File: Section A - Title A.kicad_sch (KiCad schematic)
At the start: 37 parts, among them Q1 SI2303CDS-T1-GE3, U1 AD7190WBRUZ, Y2 CSTCR4M91G53-R0

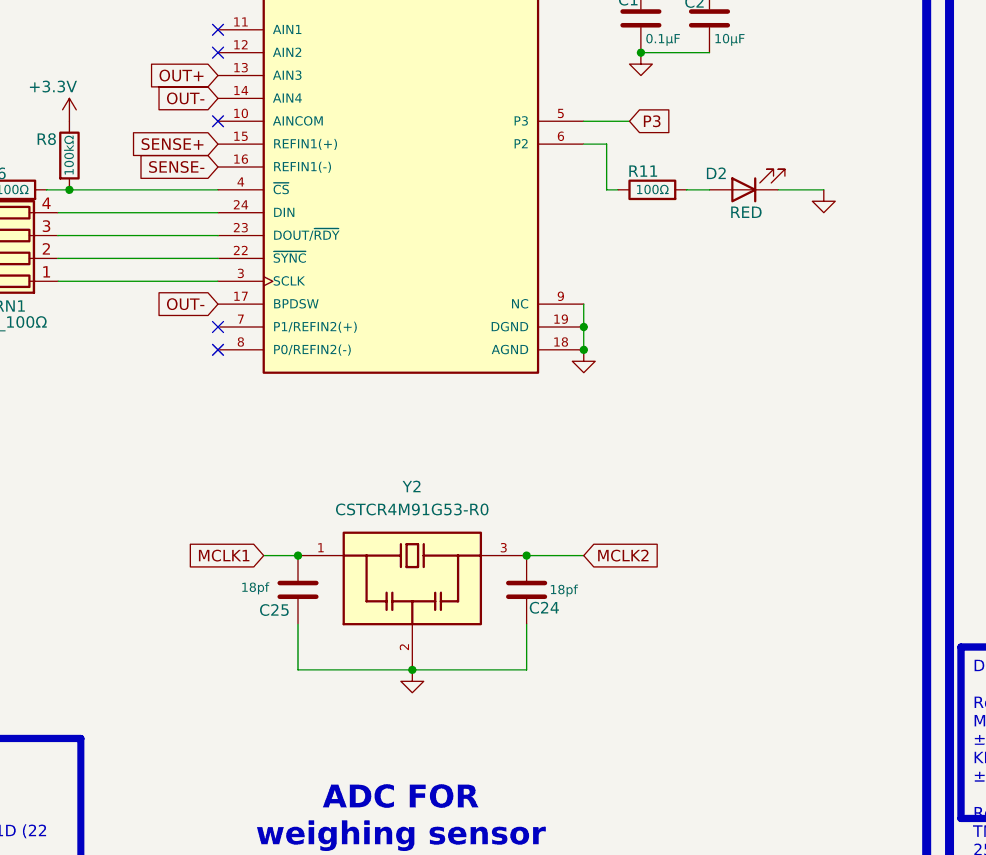
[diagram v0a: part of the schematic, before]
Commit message: [PCB V3]
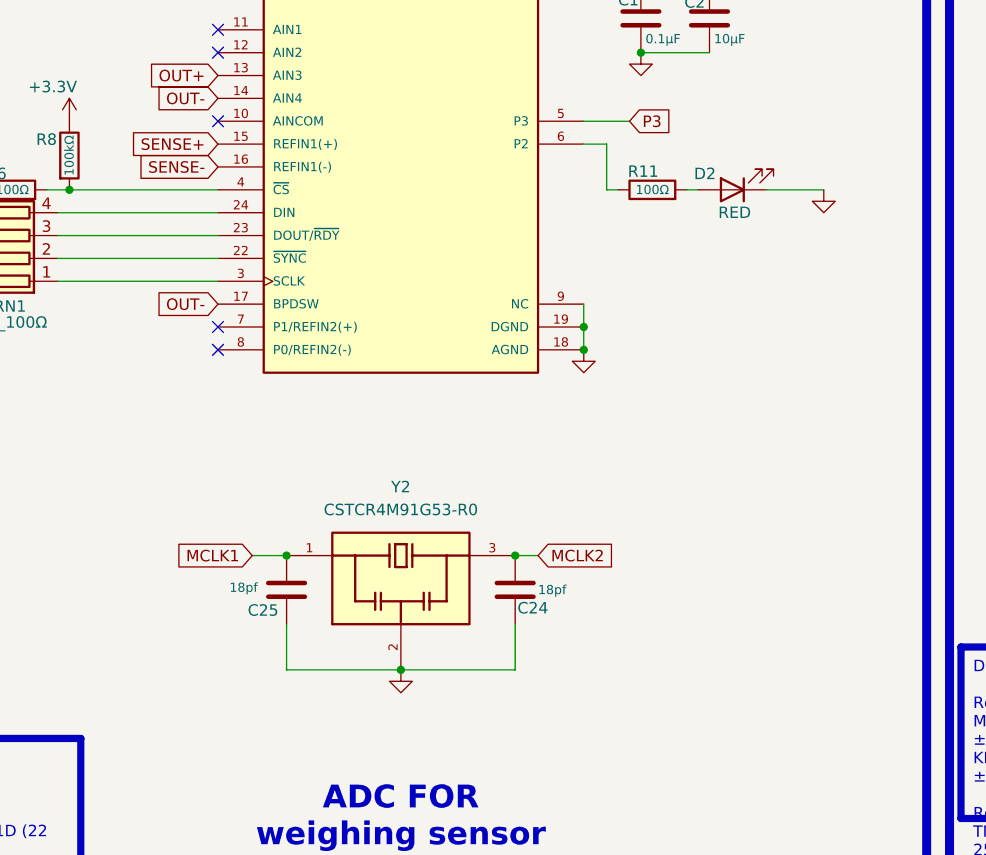
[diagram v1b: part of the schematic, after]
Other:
- moved on the sheet: C24, C25, D2, Y2
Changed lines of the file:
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@@
 	)
 	(junction
-		(at 100.33 125.73)
+		(at 99.06 125.73)
 		(diameter 0)
 		(color 0 0 0 0)
@@
 	)
 	(junction
-		(at 113.03 113.03)
+		(at 111.76 113.03)
 		(diameter 0)
 		(color 0 0 0 0)
@@
 	)
 	(junction
-		(at 87.63 113.03)
+		(at 86.36 113.03)
 		(diameter 0)
 		(color 0 0 0 0)
@@
 	(wire
 		(pts
-			(xy 119.38 113.03) (xy 113.03 113.03)
+			(xy 114.3 113.03) (xy 111.76 113.03)
 		)
 		(stroke
@@
 	(wire
 		(pts
-			(xy 113.03 125.73) (xy 100.33 125.73)
+			(xy 111.76 125.73) (xy 99.06 125.73)
 		)
 		(stroke
@@
 	(wire
 		(pts
-			(xy 113.03 120.65) (xy 113.03 125.73)
+			(xy 111.76 120.65) (xy 111.76 125.73)
 		)
 		(stroke
@@
 	(wire
 		(pts
-			(xy 87.63 120.65) (xy 87.63 125.73)
+			(xy 86.36 120.65) (xy 86.36 125.73)
 		)
 		(stroke
@@
 	(wire
 		(pts
-			(xy 130.81 72.39) (xy 133.35 72.39)
+			(xy 130.81 72.39) (xy 132.08 72.39)
 		)
 		(stroke
@@
 	(wire
 		(pts
-			(xy 83.82 113.03) (xy 87.63 113.03)
+			(xy 82.55 113.03) (xy 86.36 113.03)
 		)
 		(stroke
@@
 	(wire
 		(pts
-			(xy 140.97 72.39) (xy 146.05 72.39)
+			(xy 139.7 72.39) (xy 146.05 72.39)
 		)
 		(stroke
@@
 	(wire
 		(pts
-			(xy 87.63 125.73) (xy 100.33 125.73)
+			(xy 86.36 125.73) (xy 99.06 125.73)
 		)
 		(stroke
@@
 	(global_label "MCLK1"
 		(shape input)
-		(at 83.82 113.03 180)
+		(at 82.55 113.03 180)
 		(fields_autoplaced yes)
 		(effects
@@
 		)
 		(property "Intersheetrefs" "${INTERSHEET_REFS}"
-			(at 74.6058 113.03 0)
+			(at 73.3358 113.03 0)
 			(effects
 				(font
@@
 	(global_label "MCLK2"
 		(shape input)
-		(at 119.38 113.03 0)
+		(at 114.3 113.03 0)
 		(fields_autoplaced yes)
 		(effects
@@
 		)
 		(property "Intersheetrefs" "${INTERSHEET_REFS}"
-			(at 128.5942 113.03 0)
+			(at 123.5142 113.03 0)
 			(effects
 				(font
@@
 	(symbol
 		(lib_id "Device:C")
-		(at 113.03 116.84 0)
+		(at 111.76 116.84 0)
 		(unit 1)
 		(exclude_from_sim no)
@@
 		(dnp no)
 		(property "Reference" "C24"
-			(at 113.284 118.872 0)
+			(at 112.014 118.872 0)
 			(effects
 				(font
@@
 		)
 		(property "Value" "18pf"
-			(at 115.57 116.84 0)
+			(at 114.3 116.84 0)
 			(effects
 				(font
@@
 		)
 		(property "Footprint" "Capacitor_SMD:C_0603_1608Metric"
-			(at 113.9952 120.65 0)
+			(at 112.7252 120.65 0)
 			(effects
 				(font
@@
 		)
 		(property "Datasheet" "~"
-			(at 113.03 116.84 0)
+			(at 111.76 116.84 0)
 			(effects
 				(font
@@
 		)
 		(property "Description" "Unpolarized capacitor"
-			(at 113.03 116.84 0)
+			(at 111.76 116.84 0)
 			(effects
 				(font
@@
 	(symbol
 		(lib_id "CSTCR4M91G53-R0:CSTCR4M91G53-R0")
-		(at 100.33 115.57 0)
+		(at 99.06 115.57 0)
 		(unit 1)
 		(exclude_from_sim no)
@@
 		(fields_autoplaced yes)
 		(property "Reference" "Y2"
-			(at 100.33 105.41 0)
+			(at 99.06 105.41 0)
 			(effects
 				(font
@@
 		)
 		(property "Value" "CSTCR4M91G53-R0"
-			(at 100.33 107.95 0)
+			(at 99.06 107.95 0)
 			(effects
 				(font
@@
 		)
 		(property "Footprint" "CSTCR4M91G53-R0:OSC_CSTCR4M91G53-R0"
-			(at 100.33 115.57 0)
+			(at 99.06 115.57 0)
 			(effects
 				(font
@@
 		)
 		(property "Datasheet" ""
-			(at 100.33 115.57 0)
+			(at 99.06 115.57 0)
 			(effects
 				(font
@@
 		)
 		(property "Description" ""
-			(at 100.33 115.57 0)
+			(at 99.06 115.57 0)
 			(effects
 				(font
@@
 		)
 		(property "MF" "Murata Electronics"
-			(at 100.33 115.57 0)
+			(at 99.06 115.57 0)
 			(effects
 				(font
@@
 		)
 		(property "MAXIMUM_PACKAGE_HEIGHT" "1.2mm"
-			(at 100.33 115.57 0)
+			(at 99.06 115.57 0)
 			(effects
 				(font
@@
 		)
 		(property "Package" "SMD-3 Murata"
-			(at 100.33 115.57 0)
+			(at 99.06 115.57 0)
 			(effects
 				(font
@@
 		)
 		(property "Price" "None"
-			(at 100.33 115.57 0)
+			(at 99.06 115.57 0)
 			(effects
 				(font
@@
 		)
 		(property "Check_prices" "https://www.snapeda.com/parts/CSTCR4M91G53-R0/Murata+Electronics+North+America/view-part/?ref=eda"
-			(at 100.33 115.57 0)
+			(at 99.06 115.57 0)
 			(effects
 				(font
@@
 		)
 		(property "STANDARD" "Manufacturer Recomendations"
-			(at 100.33 115.57 0)
+			(at 99.06 115.57 0)
 			(effects
 				(font
@@
 		)
 		(property "PARTREV" "JGC42-8797"
-			(at 100.33 115.57 0)
+			(at 99.06 115.57 0)
 			(effects
 				(font
@@
 		)
 		(property "SnapEDA_Link" "https://www.snapeda.com/parts/CSTCR4M91G53-R0/Murata+Electronics+North+America/view-part/?ref=snap"
-			(at 100.33 115.57 0)
+			(at 99.06 115.57 0)
 			(effects
 				(font
@@
 		)
 		(property "MP" "CSTCR4M91G53-R0"
-			(at 100.33 115.57 0)
+			(at 99.06 115.57 0)
 			(effects
 				(font
@@
 		)
 		(property "Purchase-URL" "https://www.snapeda.com/api/url_track_click_mouser/?unipart_id=50325&manufacturer=Murata Electronics&part_name=CSTCR4M91G53-R0&search_term=cstcr4m91g53-r0"
-			(at 100.33 115.57 0)
+			(at 99.06 115.57 0)
 			(effects
 				(font
@@
 		)
 		(property "Description_1" "4.91 MHz Ceramic Resonator Built in Capacitor 15 pF ±0.2% 60 Ohms -20°C ~ 80°C Surface Mount"
-			(at 100.33 115.57 0)
+			(at 99.06 115.57 0)
 			(effects
 				(font
@@
 		)
 		(property "Availability" "In Stock"
-			(at 100.33 115.57 0)
+			(at 99.06 115.57 0)
 			(effects
 				(font
@@
 		)
 		(property "MANUFACTURER" "Murata"
-			(at 100.33 115.57 0)
+			(at 99.06 115.57 0)
 			(effects
 				(font
@@
 	(symbol
 		(lib_id "power:GND")
-		(at 100.33 125.73 0)
+		(at 99.06 125.73 0)
 		(unit 1)
 		(exclude_from_sim no)
@@
 		(fields_autoplaced yes)
 		(property "Reference" "#PWR013"
-			(at 100.33 132.08 0)
+			(at 99.06 132.08 0)
 			(effects
 				(font
@@
 		)
 		(property "Value" "GND"
-			(at 100.33 130.81 0)
+			(at 99.06 130.81 0)
 			(effects
 				(font
@@
 		)
 		(property "Footprint" ""
-			(at 100.33 125.73 0)
+			(at 99.06 125.73 0)
 			(effects
 				(font
@@
 		)
 		(property "Datasheet" ""
-			(at 100.33 125.73 0)
+			(at 99.06 125.73 0)
 			(effects
 				(font
@@
 		)
 		(property "Description" "Power symbol creates a global label with name \"GND\" , ground"
-			(at 100.33 125.73 0)
+			(at 99.06 125.73 0)
 			(effects
 				(font
@@
 	(symbol
 		(lib_id "Device:C")
-		(at 87.63 116.84 0)
+		(at 86.36 116.84 0)
 		(unit 1)
 		(exclude_from_sim no)
@@
 		(dnp no)
 		(property "Reference" "C25"
-			(at 83.312 119.126 0)
+			(at 82.042 119.126 0)
 			(effects
 				(font
@@
 		)
 		(property "Value" "18pf"
-			(at 81.28 116.586 0)
+			(at 80.01 116.586 0)
 			(effects
 				(font
@@
 		)
 		(property "Footprint" "Capacitor_SMD:C_0603_1608Metric"
-			(at 88.5952 120.65 0)
+			(at 87.3252 120.65 0)
 			(effects
 				(font
@@
 		)
 		(property "Datasheet" "~"
-			(at 87.63 116.84 0)
+			(at 86.36 116.84 0)
 			(effects
 				(font
@@
 		)
 		(property "Description" "Unpolarized capacitor"
-			(at 87.63 116.84 0)
+			(at 86.36 116.84 0)
 			(effects
 				(font
@@
 	(symbol
 		(lib_id "Device:LED")
-		(at 137.16 72.39 180)
+		(at 135.89 72.39 180)
 		(unit 1)
 		(exclude_from_sim no)
@@
 		(dnp no)
 		(property "Reference" "D2"
-			(at 134.112 70.612 0)
+			(at 132.842 70.612 0)
 			(effects
 				(font
@@
 		)
 		(property "Value" "RED"
-			(at 137.414 74.93 0)
+			(at 136.144 74.93 0)
 			(effects
 				(font
@@
 		)
 		(property "Footprint" "LED_SMD:LED_0603_1608Metric"
-			(at 137.16 72.39 0)
+			(at 135.89 72.39 0)
 			(effects
 				(font
@@
 		)
 		(property "Datasheet" "~"
-			(at 137.16 72.39 0)
+			(at 135.89 72.39 0)
 			(effects
 				(font
@@
 		)
 		(property "Description" "Light emitting diode"
-			(at 137.16 72.39 0)
+			(at 135.89 72.39 0)
 			(effects
 				(font
@@
 		)
 		(property "Sim.Pins" "1=K 2=A"
-			(at 137.16 72.39 0)
+			(at 135.89 72.39 0)
 			(effects
 				(font
